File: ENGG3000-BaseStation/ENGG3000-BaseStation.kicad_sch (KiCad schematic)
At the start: 49 parts, among them J2 OLED, J3 Buttons, J4 USB_C_Receptacle_USB2.0_16P, J5 Cell 3, J6 Cell 2, J7 Cell 1, J8 CHRG LED, Q1 SS8050, Q2 AO3401A, SW1 RESET, SW2 BOOT, U1 ESP32-S3-WROOM-1-N16R8, U2 CN3085, U3 TPS63001DRCR

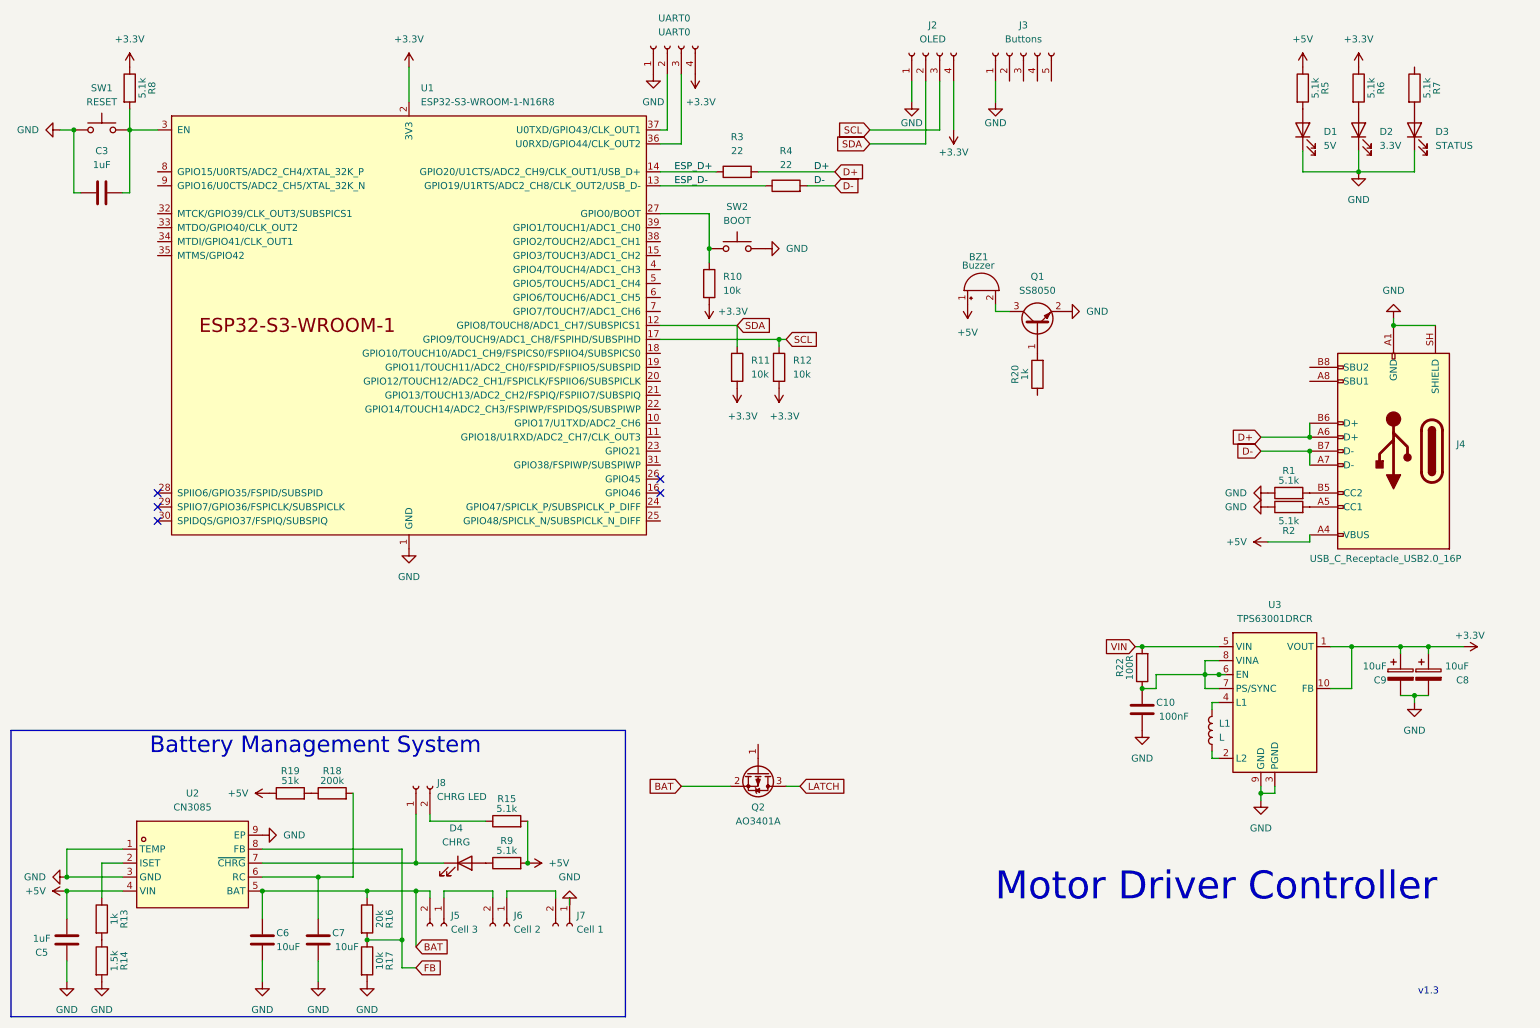
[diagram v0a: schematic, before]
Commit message: Updated power path
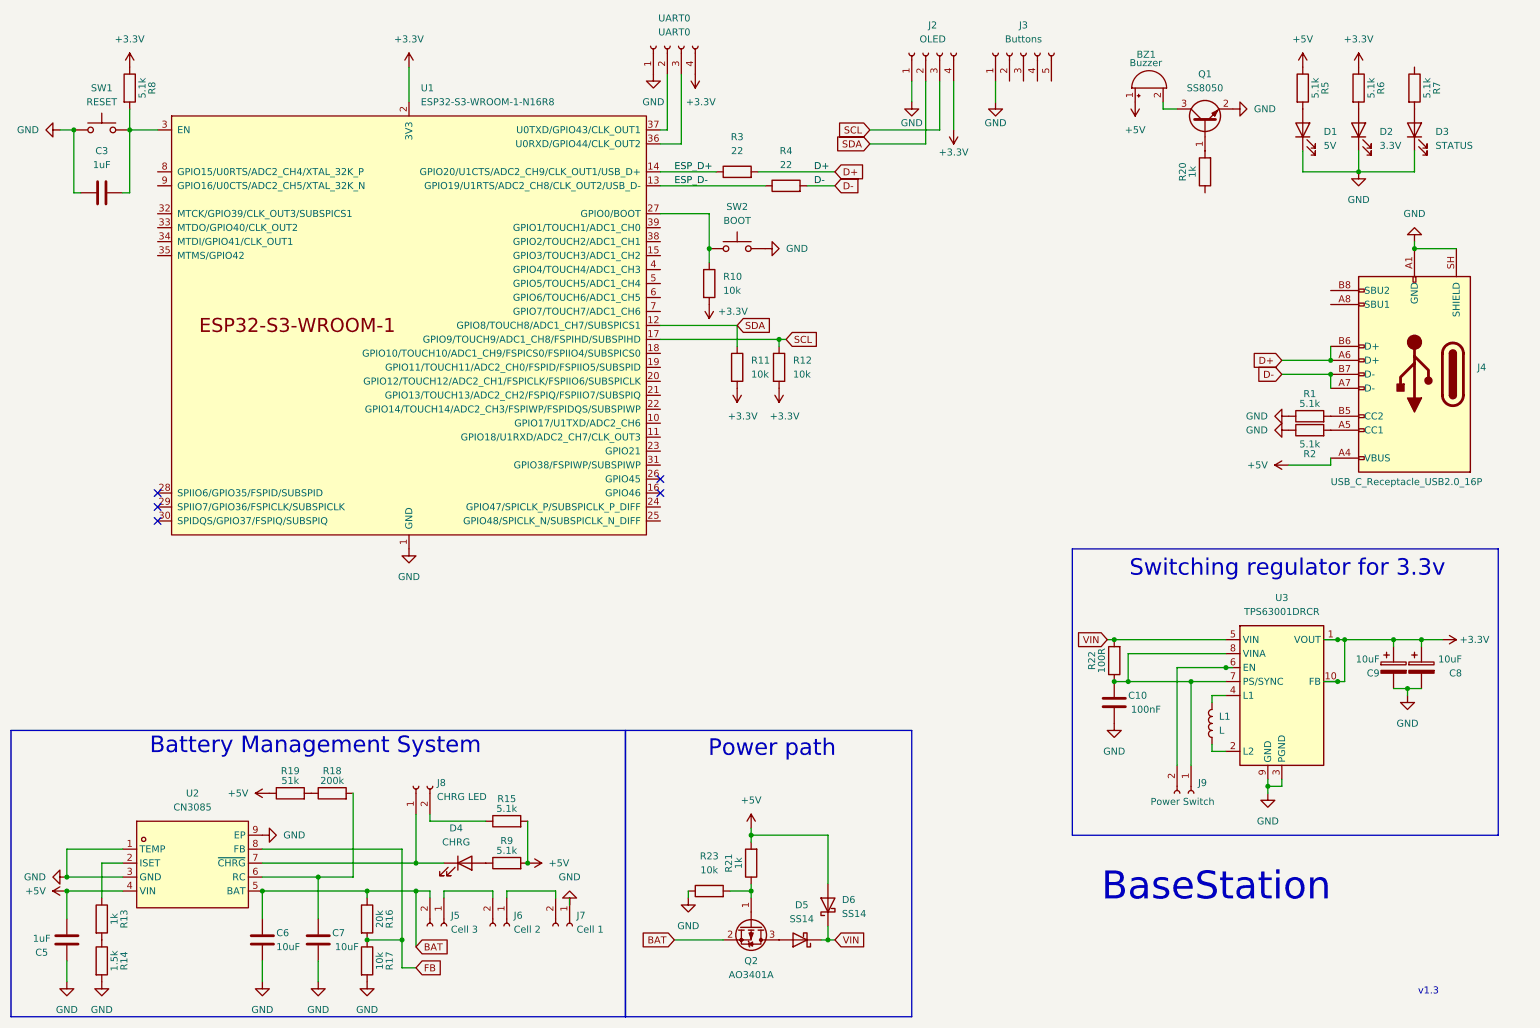
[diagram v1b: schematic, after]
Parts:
- added D5, D6: SS14, Diode_SMD:D_SMA, symbol Diode:SS14
- added J9: Power Switch, Connector_JST:JST_XH_B2B-XH-A_1x02_P2.50mm_Vertical, symbol Connector:Conn_01x02_Socket
- added R21: 1k, Resistor_SMD:R_0402_1005Metric, symbol Device:R
- added R23: 10k, Resistor_SMD:R_0402_1005Metric, symbol Device:R
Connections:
- net +5V: now also D6.2 (A), R21.2
- net GND: now also R23.1
- net VIN: now also D5.1 (K), D6.1 (K)
- net at C10.1, R22.1, U3.7 (PS/SYNC)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: now also J9.1 (-); no longer U3.6 (EN)
- net at Q2.1 (G): now also R21.1, R23.2
- net LATCH: no longer names the net of Q2.3 (D)
- net LATCH: now also D5.2 (A)
- new net: J9.2 (+), U3.6 (EN)
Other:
- note added: "BaseStation"
- note added: "Power path"
- note added: "Switching regulator for 3.3v"
- note removed: "Motor Driver Controller"
- moved on the sheet: BZ1, C10, C8, C9, J4, L1, Q1, Q2, R1, R2, R20, R22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
